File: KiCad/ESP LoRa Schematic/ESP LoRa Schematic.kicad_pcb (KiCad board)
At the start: 2 copper layers, 106 x 60 mm, 12 parts, among them J1 Conn_01x05_Socket, J2 Conn_01x02_Socket, U1 ESP32-S3-DEVKITC-1-N8R8, U2 RA-02_LORA

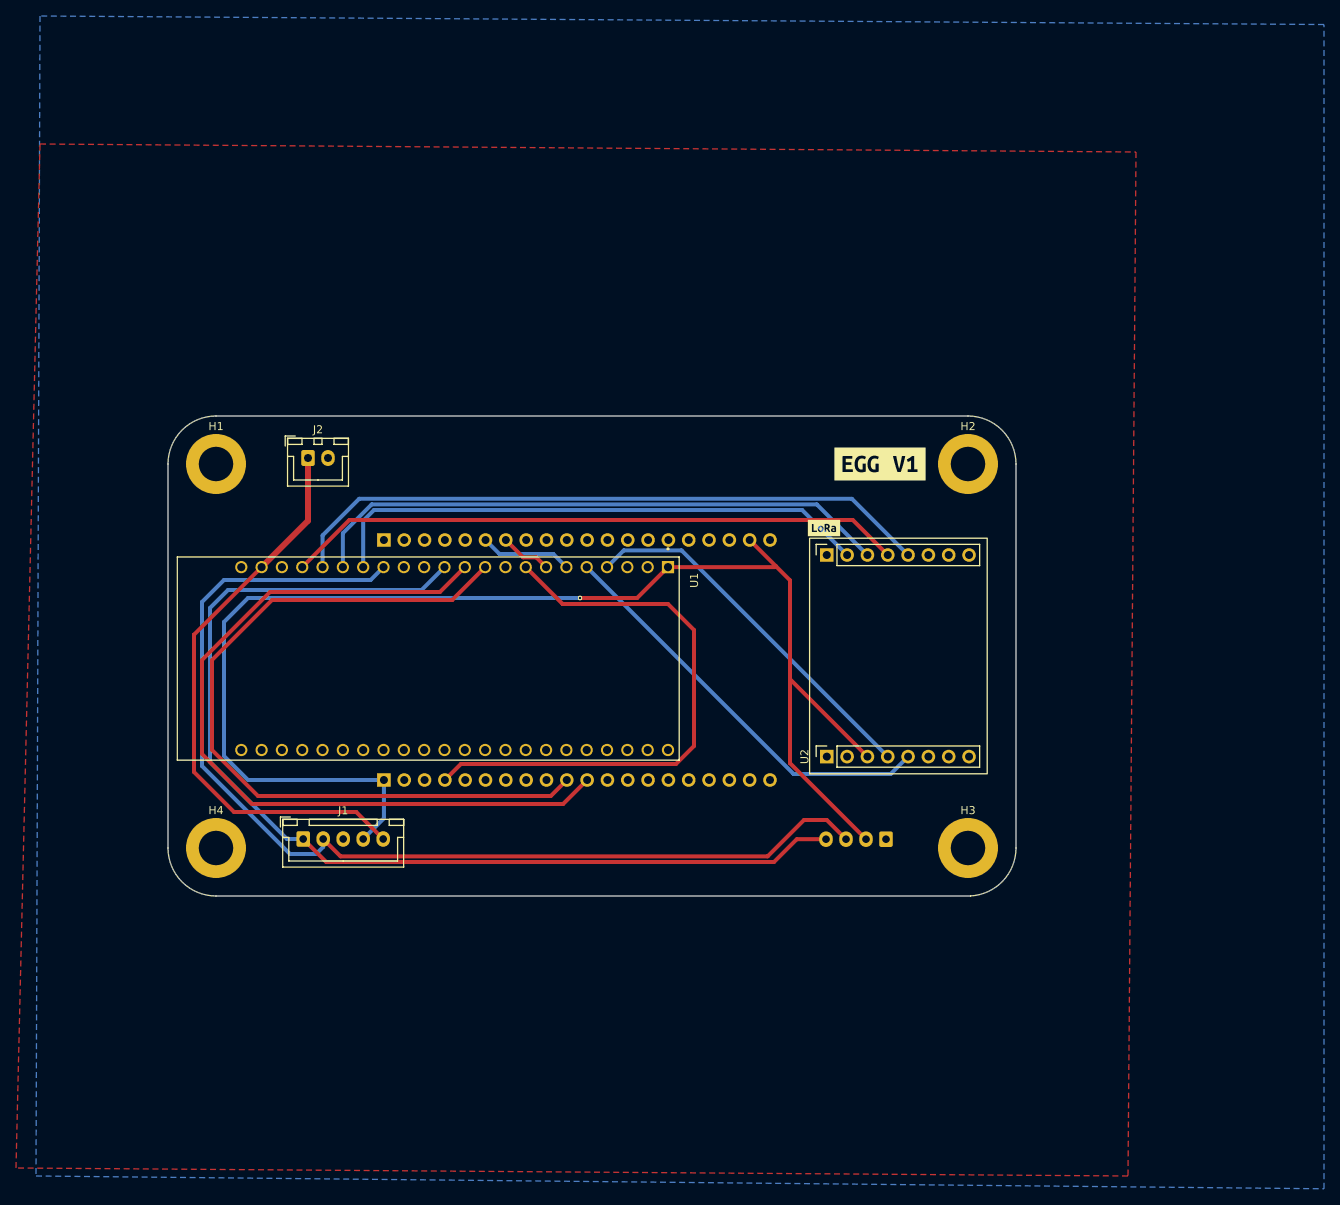
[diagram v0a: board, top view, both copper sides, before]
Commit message: New Egg Folder
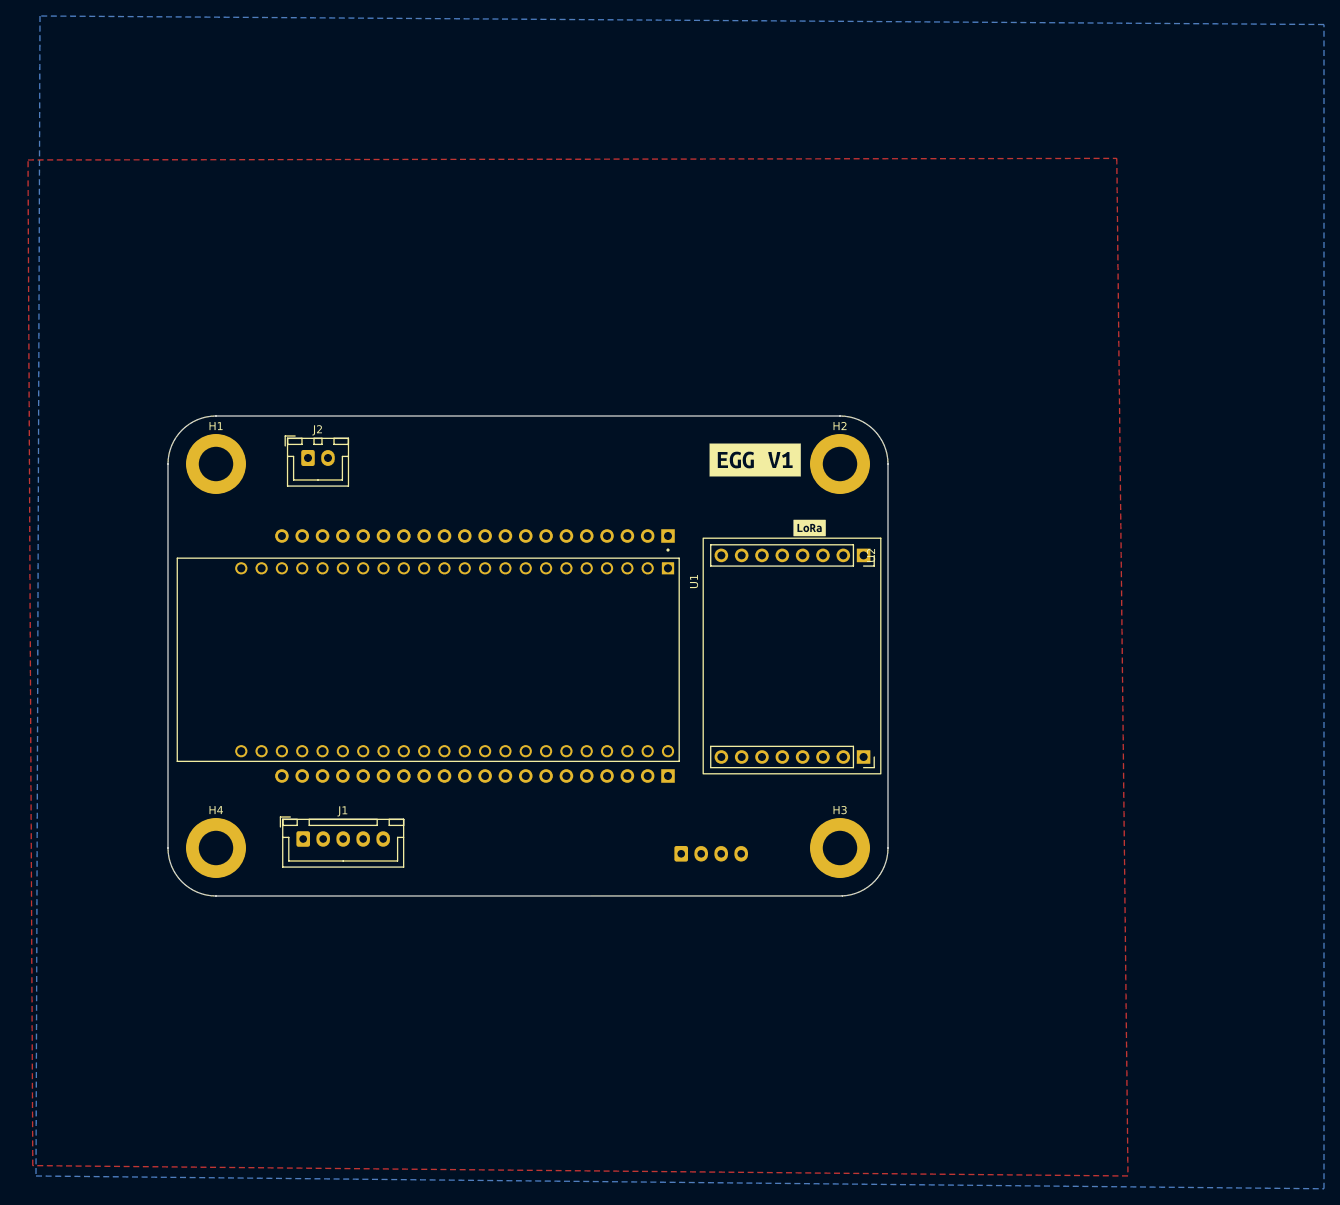
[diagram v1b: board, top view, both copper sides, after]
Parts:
- moved U3 49.0 mm to (134.3, 111.0), turned to 90 degrees
- moved OLED1 25.7 mm to (134.2, 120.7), turned to 0 degrees
- moved U2 25.6 mm to (156.9, 83.4), turned to -90 degrees
- moved H2 16.0 mm to (154.0, 72.0)
- moved H3 16.0 mm to (154.0, 120.0)
- moved kibuzzard-69B7B2E3 15.6 mm to (143.4, 71.5)
- moved kibuzzard-69B7B320 1.80 mm to (150.2, 80.0)
- moved U1 0.15 mm to (102.5, 96.5)
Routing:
- net +3.3V: track 176.0 -> 0.00 mm, vias 1 -> 0
- net GPIO9: track 135.2 -> 0.00 mm
- net GPIO8: track 134.0 -> 0.00 mm
- net GPIO18: track 101.4 -> 0.00 mm
- net GPIO17: track 97.8 -> 0.00 mm
- net GPIO12: track 82.0 -> 0.00 mm
- net GPIO13: track 77.4 -> 0.00 mm
- net GPIO11: track 73.9 -> 0.00 mm
- net +5V: track 72.3 -> 0.28 mm
- net GPIO15: track 71.7 -> 0.00 mm
- net GPIO10: track 69.2 -> 0.00 mm
- net GPIO5: track 51.8 -> 0.00 mm
- net GPIO4: track 46.6 -> 0.00 mm
- net GPIO6: track 11.5 -> 0.00 mm
- net GPIO7: track 6.43 -> 0.00 mm
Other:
- board size 106 x 60 mm -> 90 x 60 mm
